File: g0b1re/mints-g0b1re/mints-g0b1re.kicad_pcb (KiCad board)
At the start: 2 copper layers, 162 parts, among them J1 Conn_01x08, J3 Conn_01x02, J4 Conn_01x04, J5 Conn_01x04, J6 FTSH-107-01-X-DV-K, J7 Conn_01x04, Q1 SQM120P06-07L_GE3, Q2 SQM120P06-07L_GE3, Q3 SQM120P06-07L_GE3, Q4 SQM120P06-07L_GE3, Q5 SQM120P06-07L_GE3, Q6 SQM120P06-07L_GE3, Q7 SQM120P06-07L_GE3, Q8 SQM120P06-07L_GE3, SW1 SW_Coded_SH-7050, U1 STM32G0B1RETx, U2 TCAN3414DDFR, U201 140357145200, U202 140357145200, U203 140357145200, U204 140357145200, U205 140357145200, U206 140357145200, U207 140357145200, U208 140357145200, U3 MCP3564R, U4 TCA9548, U5 AP63203WU, U6 LM4040CIM3-2.0/NOPB

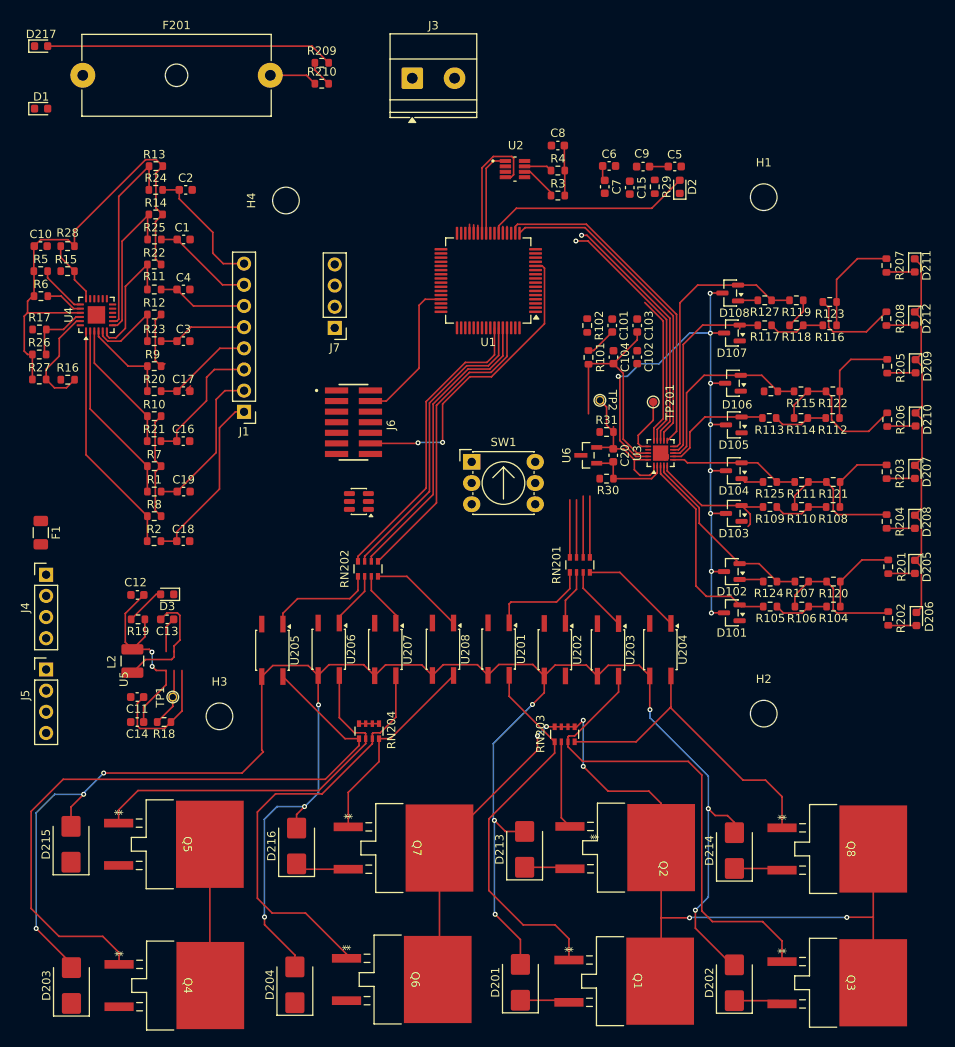
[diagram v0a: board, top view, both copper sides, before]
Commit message: board updates 9/2/26
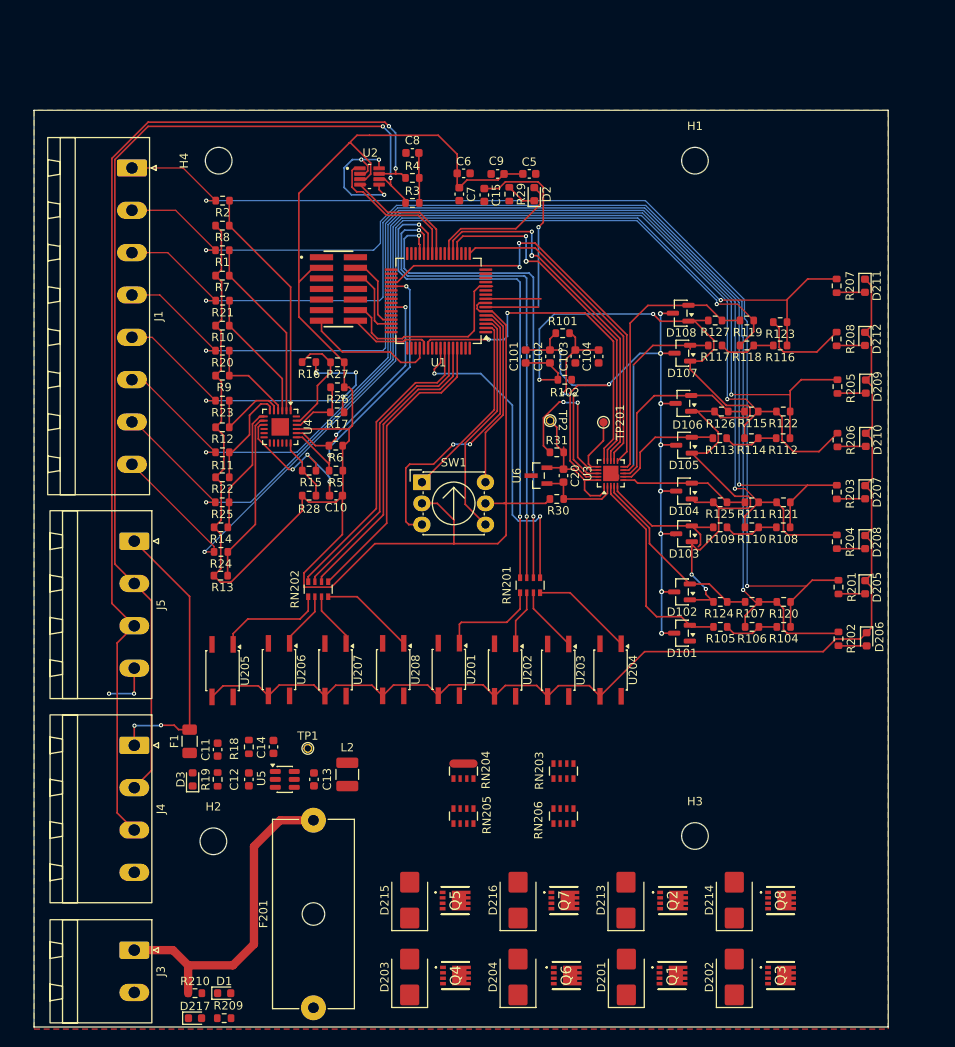
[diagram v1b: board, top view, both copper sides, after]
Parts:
- removed C1, C16, C17, C18, C19, C2, C3, C4: 10n, Capacitor_SMD:C_0603_1608Metric
- removed J7: Conn_01x04, Connector_PinHeader_2.54mm:PinHeader_1x04_P2.54mm_Vertical
- added RN205: 5k1, Resistor_SMD:R_Array_Convex_4x0603, F.Cu at (138.5, 184.7)
- added RN206: 5k1, Resistor_SMD:R_Array_Convex_4x0603, F.Cu at (126.5, 184.7)
- J1: footprint Connector_PinHeader_2.54mm:PinHeader_1x08_P2.54mm_Vertical -> Connector_Phoenix_MSTB:PhoenixContact_MSTBA_2,5_8-G-5,08_1x08_P5.08mm_Horizontal
- J3: footprint TerminalBlock_Phoenix:TerminalBlock_Phoenix_MKDS-1,5-2-5.08_1x02_P5.08mm_Horizontal -> Connector_Phoenix_MSTB:PhoenixContact_MSTBA_2,5_2-G-5,08_1x02_P5.08mm_Horizontal
- J4, J5: footprint Connector_PinHeader_2.54mm:PinHeader_1x04_P2.54mm_Vertical -> Connector_Phoenix_MSTB:PhoenixContact_MSTBA_2,5_4-G-5,08_1x04_P5.08mm_Horizontal
- Q1, Q2, Q3, Q4, Q5, Q6, Q7, Q8: footprint SQM120P06-07L_GE3:TO-263_SQM120P06-07L_GE3_VIS -> LIB_DMP6023LFGQ-7:DMTH8008LFGQ7
- moved D217 118.1 mm to (94.3, 208.9)
- moved F201 115.3 mm to (108.5, 207.7), turned to 90 degrees
- moved R209 115.2 mm to (97.8, 208.9), turned to 180 degrees
- moved R210 110.2 mm to (94.3, 205.9)
- moved J3 109.8 mm to (87.0, 200.8), turned to -90 degrees
- moved D1 108.4 mm to (97.8, 205.9)
- moved H2 67.8 mm to (96.5, 187.7)
- moved H3 58.8 mm to (154.3, 187.1)
- moved R13 49.8 mm to (97.4, 155.8), turned to 0 degrees
- moved C10 46.4 mm to (111.2, 146.2), turned to 180 degrees
- moved R24 44.1 mm to (97.4, 153.0), turned to 180 degrees
- moved R5 42.8 mm to (111.2, 143.2), turned to 180 degrees
- moved R2 41.7 mm to (97.6, 110.8), turned to 180 degrees
- moved R28 41.7 mm to (108.0, 146.2), turned to 0 degrees
- moved D215 41.2 mm to (120.1, 194.8)
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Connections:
- Q1 pad 1: /outputs/~{ISO_OUT_0} -> Net-(Q1-G)
- Q2 pad 1: /outputs/~{ISO_OUT_1} -> Net-(Q2-G)
- Q3 pad 1: /outputs/~{ISO_OUT_2} -> unconnected-(Q3-G-Pad1)
- Q4 pad 1: /outputs/~{ISO_OUT_4} -> Net-(Q4-G)
- Q5 pad 1: /outputs/~{ISO_OUT_5} -> Net-(Q5-G)
- Q6 pad 1: /outputs/~{ISO_OUT_6} -> Net-(Q6-G)
- Q7 pad 1: /outputs/~{ISO_OUT_7} -> Net-(Q7-G)
- Q8 pad 1: /outputs/~{ISO_OUT_3} -> Net-(Q8-G)
- R3 pad 1: CAN + -> CAN+
- R4 pad 1: CAN - -> CAN-
- RN203 pad 5: /outputs/~{ISO_OUT_0} -> Net-(Q1-G)
- RN203 pad 6: /outputs/~{ISO_OUT_1} -> Net-(Q2-G)
- RN203 pad 7: /outputs/~{ISO_OUT_2} -> Net-(RN203B-R2.2)
- RN203 pad 8: /outputs/~{ISO_OUT_3} -> Net-(Q8-G)
- RN204 pad 5: /outputs/~{ISO_OUT_4} -> Net-(Q4-G)
- RN204 pad 6: /outputs/~{ISO_OUT_5} -> Net-(Q5-G)
- RN204 pad 7: /outputs/~{ISO_OUT_6} -> Net-(Q6-G)
- RN204 pad 8: /outputs/~{ISO_OUT_7} -> Net-(Q7-G)
- U2 pad 6: CAN + -> CAN+
- U2 pad 7: CAN - -> CAN-
- U203 pad 4: /outputs/~{ISO_OUT_2} -> AUX_POW-
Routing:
- net AUX_POW-: track 297.4 -> 136.1 mm, vias 12 -> 0
- net VPOW: track 139.7 -> 2.40 mm, vias 6 -> 0
- net +3V3: track 136.0 -> 270.2 mm
- net CAN-: track 0.00 -> 128.1 mm, vias 0 -> 2
- net CAN+: track 0.00 -> 124.0 mm, vias 0 -> 2
- net OUT5/IN2-: track 28.7 -> 136.7 mm, vias 0 -> 2
- net OUT4/IN2+: track 22.6 -> 130.6 mm, vias 0 -> 2
- net OUT3/IN1-: track 34.1 -> 139.8 mm, vias 0 -> 2
- net GNDA: track 8.12 -> 108.7 mm, vias 0 -> 4
- net OUT2/IN1+: track 31.2 -> 131.6 mm, vias 0 -> 2
- net OUT6/IN3+: track 24.7 -> 125.1 mm, vias 0 -> 2
- net OUT1/IN0-: track 40.6 -> 139.5 mm, vias 0 -> 2
- net OUT0/IN0+: track 37.1 -> 133.8 mm, vias 0 -> 2
- net OUT7/IN3-: track 37.2 -> 127.8 mm, vias 0 -> 2
- net /outputs/~{ISO_OUT_4}: track 81.5 -> 0.00 mm
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- added copper zone on F.Cu, net GND
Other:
- board outline added: 102.5 x 110 mm
- board text added: "R126"
